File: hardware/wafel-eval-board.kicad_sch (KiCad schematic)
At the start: 46 parts, among them Q101 AO3422, U101 LM5163DDA

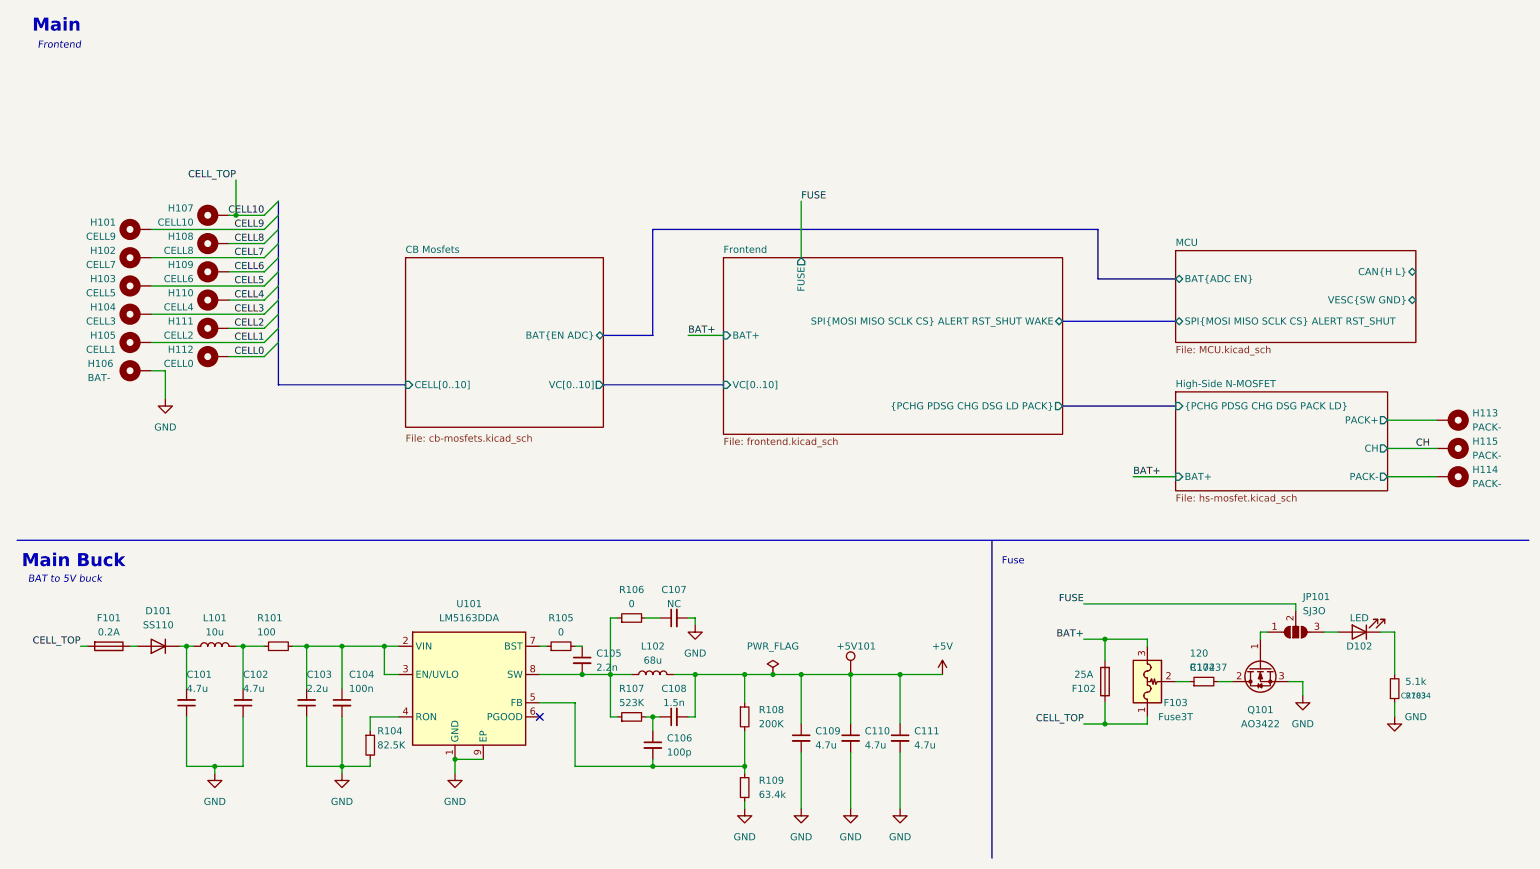
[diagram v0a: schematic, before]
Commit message: improve can
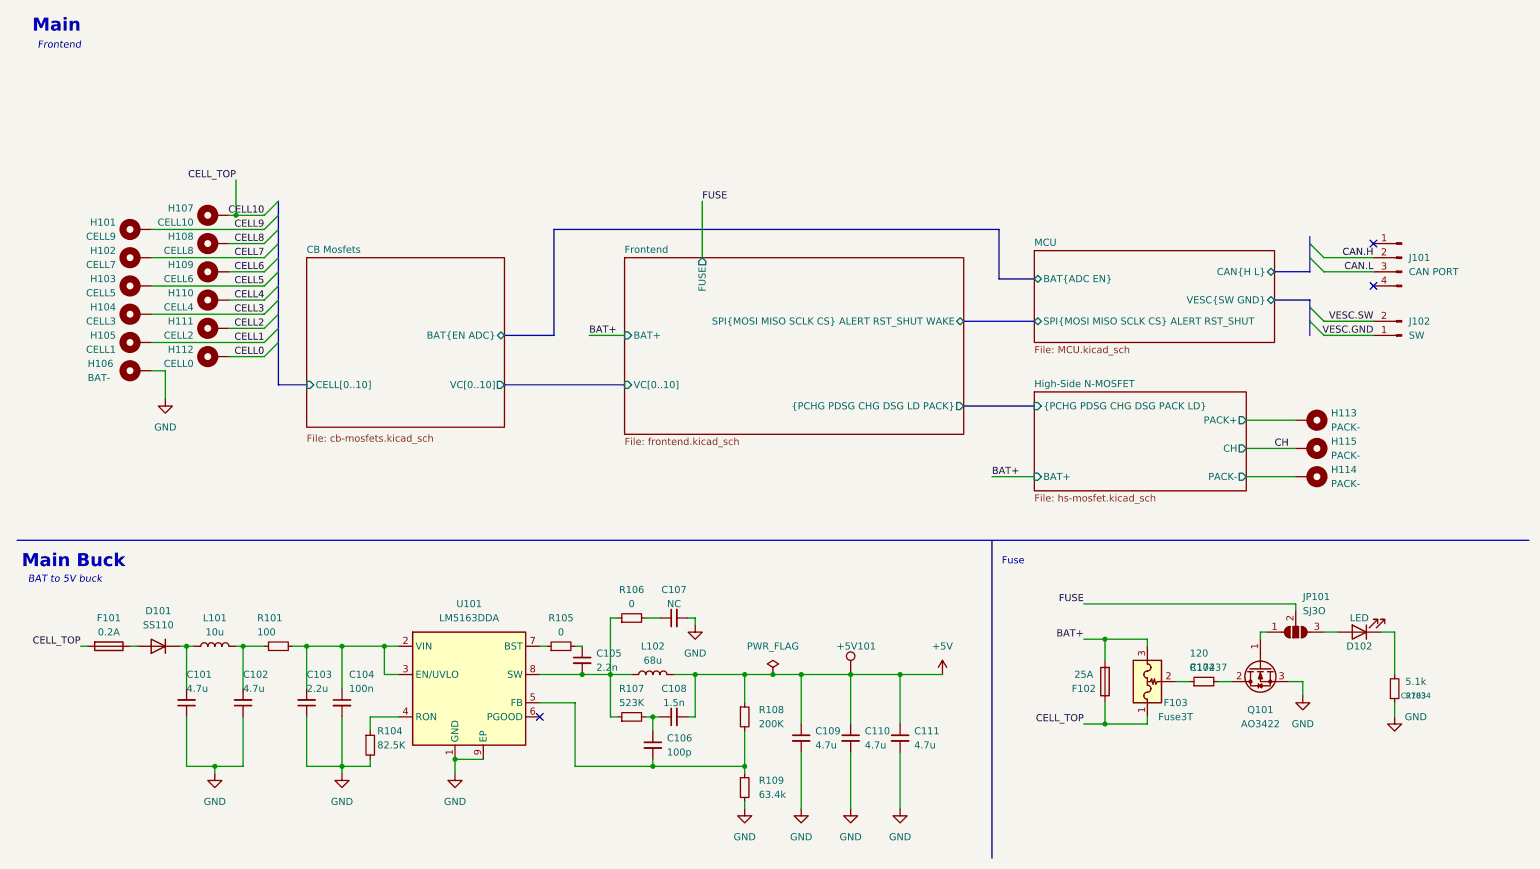
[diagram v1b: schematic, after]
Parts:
- added J101: CAN PORT, Connector_JST:JST_PH_S4B-PH-K_1x04_P2.00mm_Horizontal, symbol Connector:Conn_01x04_Pin
- added J102: SW, Connector_JST:JST_PH_S2B-PH-K_1x02_P2.00mm_Horizontal, symbol Connector:Conn_01x02_Pin
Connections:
- new net CAN.H: J101.2 (Pin_2)
- new net CAN.L: J101.3 (Pin_3)
- new net VESC.GND: J102.1 (Pin_1)
- new net VESC.SW: J102.2 (Pin_2)
- no-connect marks 1 -> 3
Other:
- moved on the sheet: H113, H114, H115
